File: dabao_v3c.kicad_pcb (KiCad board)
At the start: 2 copper layers, 21 x 41 mm, 51 parts, among them J1 USB_C_Receptacle_USB2.0_16P, SW1 SW_Push, SW2 SW_Push, U1 baochip1x, U3 Baochip, U4 MT3406, U5 EMS4000RSW, U6 MT3406, Y2 48.000MHz

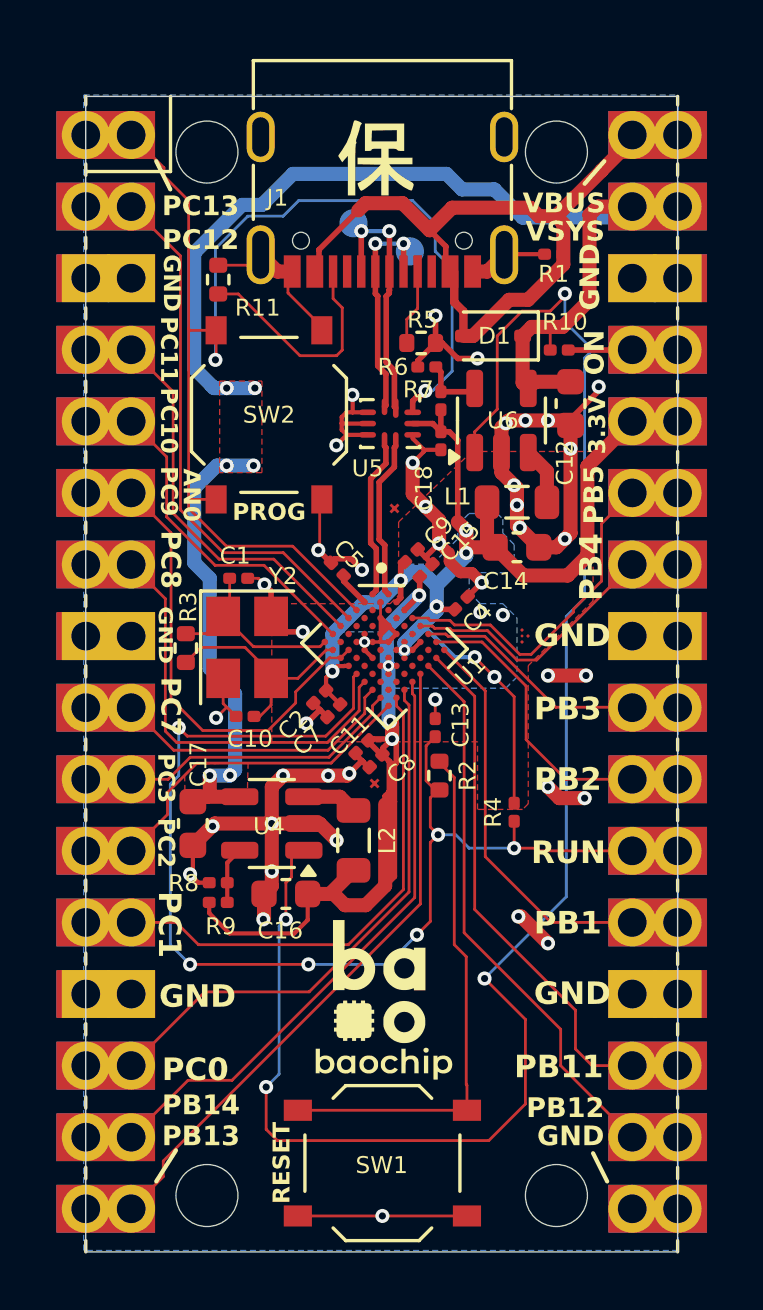
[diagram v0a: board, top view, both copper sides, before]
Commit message: initial placement
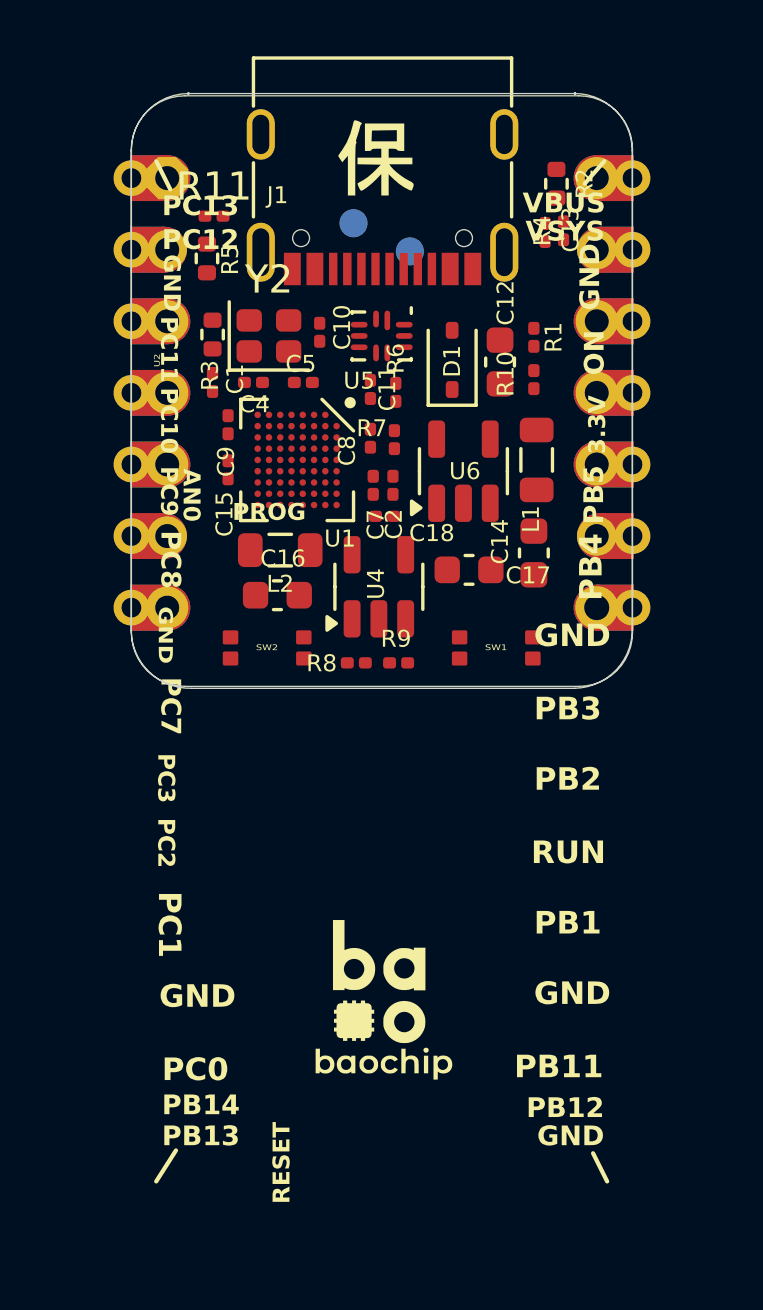
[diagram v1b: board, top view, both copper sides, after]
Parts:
- removed FID1, FID2: Fiducial, common:IRIS fiducial 0.4mm
- removed FID3: Fiducial, common:IRIS fiducial2 0.4mm
- removed H1, H2, H3, H4: MountingHole, MountingHole:MountingHole_2.2mm_M2_DIN965
- removed U3: Baochip, common:Dabao_Vendor_Substrate
- added U2: ~, xiao:MOUDLE14P-XIAO-HALF-HOLE, F.Cu at (132.0, 70.0)
- R11: footprint Resistor_SMD:R_0402_1005Metric -> Resistor_SMD:R_0201_0603Metric
- SW1, SW2: value SW_Push -> SKTAAAE010; footprint common:SW_Push_1P1T_XKB_TS-1187A -> xiao:SW4-SMD-2.8-2.6X1.6X0.53MM
- Y2: footprint Crystal:Crystal_SMD_3225-4Pin_3.2x2.5mm -> Crystal:Crystal_SMD_2016-4Pin_2.0x1.6mm
- moved R2 21.4 mm to (138.2, 62.6)
- moved R4 20.7 mm to (138.4, 64.3)
- moved SW1 18.7 mm to (136.1, 79.1), turned to 0 degrees
- moved C13 18.0 mm to (137.8, 64.3)
- moved C10 13.9 mm to (129.8, 67.9), turned to 90 degrees
- moved C17 13.3 mm to (135.1, 76.3), turned to 180 degrees
- moved C11 12.7 mm to (131.6, 69.9), turned to 90 degrees
- moved C8 11.4 mm to (131.6, 71.6), turned to 90 degrees
- moved R3 11.2 mm to (126.0, 68.0), turned to -90 degrees
- moved Y2 11.1 mm to (128.0, 68.0), turned to 0 degrees
- moved C4 10.8 mm to (127.5, 69.7), turned to 0 degrees
- moved R9 10.6 mm to (132.6, 79.6), turned to 180 degrees
- moved L2 10.6 mm to (128.4, 75.6), turned to 180 degrees
- moved C16 10.6 mm to (128.3, 77.2), turned to 0 degrees
- moved U4 9.22 mm to (131.9, 76.9), turned to 90 degrees
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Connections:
- R2 pad 1: Net-(R2-Pad1) -> Net-(SW1-B0)
- SW1 pad 1: GND -> (no net)
- SW1 pad 2: Net-(R2-Pad1) -> (no net)
- SW2 pad 1: GND -> (no net)
- SW2 pad 2: /PC13 -> (no net)
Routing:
- net GND: track 81.7 -> 0.00 mm, vias 41 -> 0
- net /EN: track 62.5 -> 0.00 mm, vias 4 -> 0
- net /VSYS: track 51.7 -> 0.00 mm, vias 6 -> 0
- net /PC13: track 45.2 -> 0.00 mm, vias 2 -> 0
- net +3.3V: track 43.1 -> 0.00 mm, vias 10 -> 0
- net /RST_N: track 41.2 -> 0.00 mm, vias 6 -> 0
- net +0.9V: track 30.7 -> 0.00 mm, vias 4 -> 0
- net VBUS: track 25.1 -> 0.00 mm
- net /PB13: track 23.2 -> 0.00 mm
- net /PB14: track 21.3 -> 0.00 mm
- net /PB12: track 19.7 -> 0.00 mm
- net /PC0: track 19.7 -> 0.00 mm
- net /PC12: track 19.0 -> 0.00 mm
- net Net-(R2-Pad1): track 18.8 -> 0.00 mm
- net /PB11: track 18.2 -> 0.00 mm
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- removed copper zone on B.Cu, net +3.3V
- removed copper zone on F.Cu, net +3.3V
- removed copper zone on F.Cu, net /VSYS
- removed copper zone on B.Cu, net GND
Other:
- board size 21 x 41 mm -> 17.8 x 21.1 mm
- copper layers 2 -> 6
